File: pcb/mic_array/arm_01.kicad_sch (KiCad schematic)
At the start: 16 parts, among them U10 IM72D128V01XTMA1, U11 IM72D128V01XTMA1, U12 IM72D128V01XTMA1, U13 IM72D128V01XTMA1, U14 IM72D128V01XTMA1, U15 IM72D128V01XTMA1, U16 IM72D128V01XTMA1, U9 IM72D128V01XTMA1

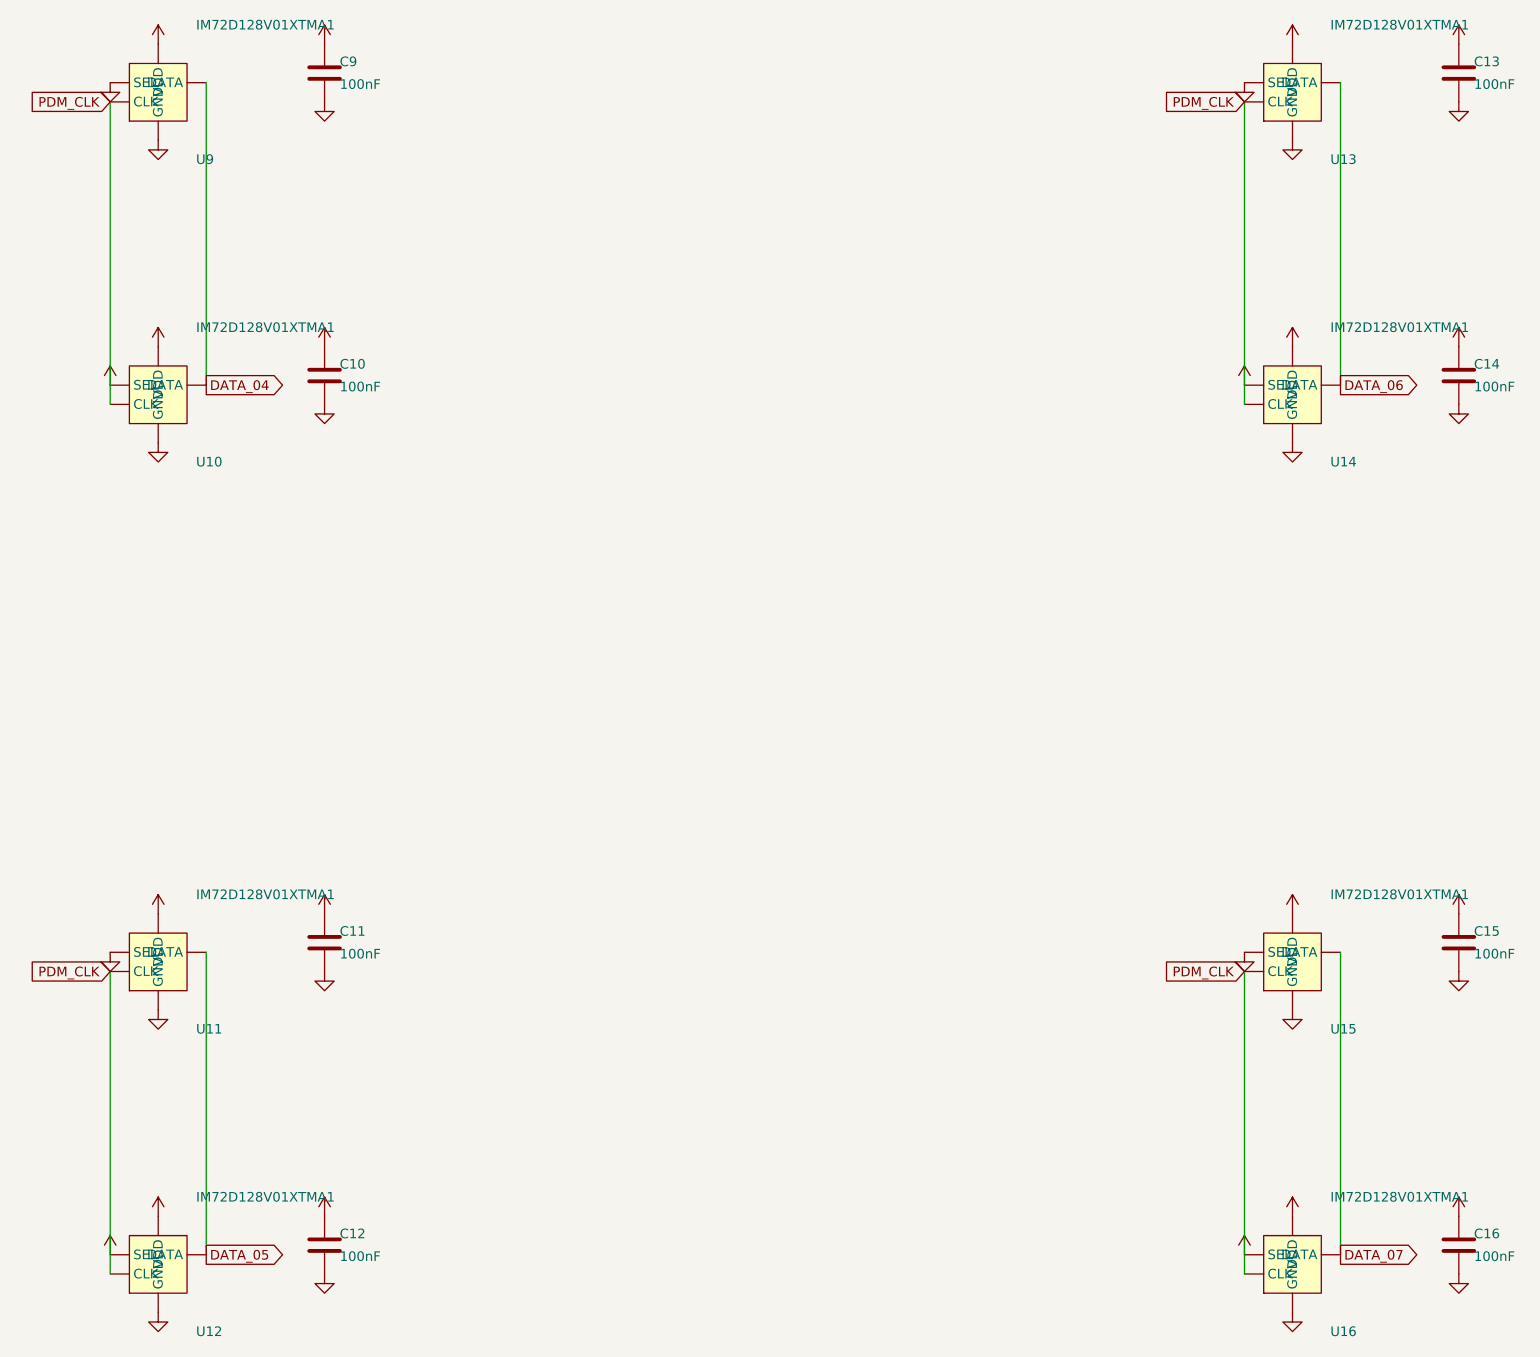
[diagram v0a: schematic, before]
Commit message: Updated.
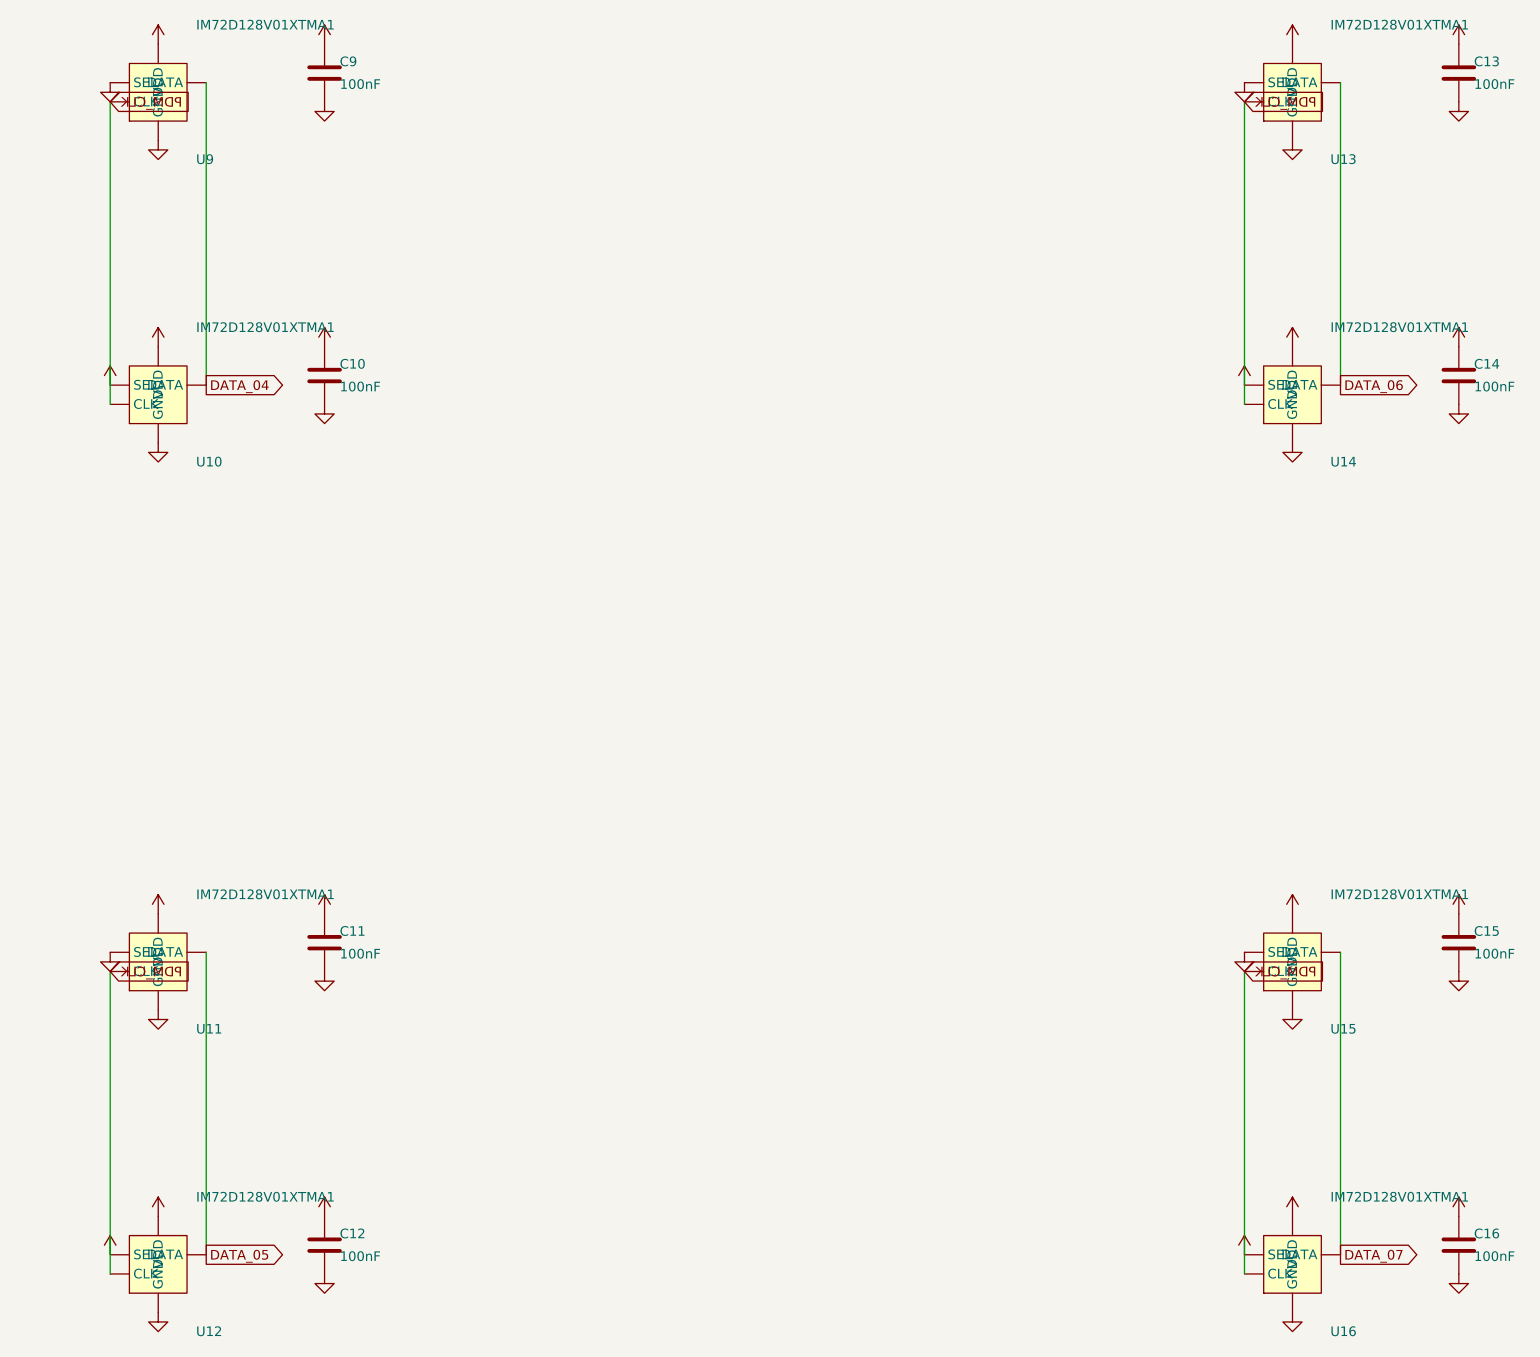
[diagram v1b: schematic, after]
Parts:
- C10, C11, C12, C13, C14, C15, C16, C9: footprint Capacitor_SMD:C_0402_1005Metric -> (none)
- U10, U11, U12, U13, U14, U15, U16, U9: footprint Sensor_Audio:Infineon_PG-LLGA-5-2 -> (none)
